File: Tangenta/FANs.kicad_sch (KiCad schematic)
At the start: 8 parts, among them M1 Fan_4pin, M2 Fan_4pin, Q3 BSS138

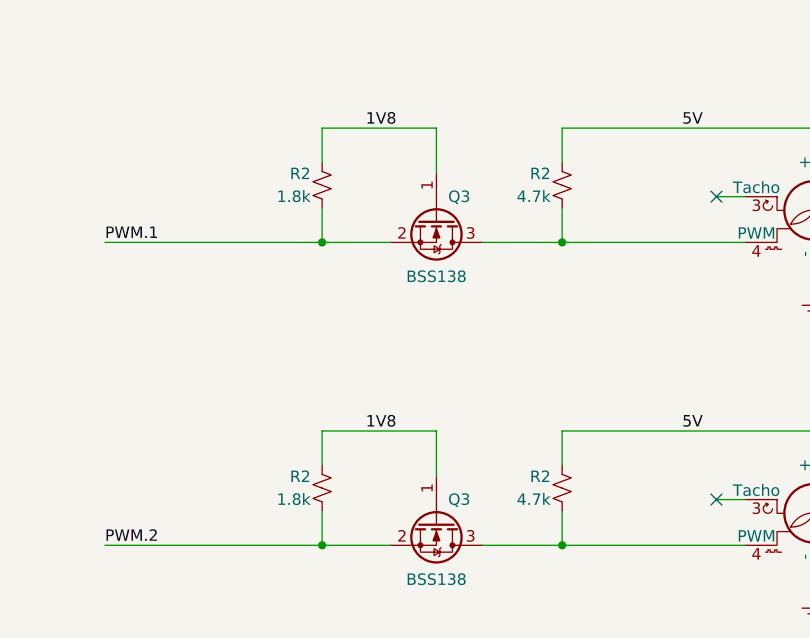
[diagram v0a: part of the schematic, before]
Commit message: initialize branch
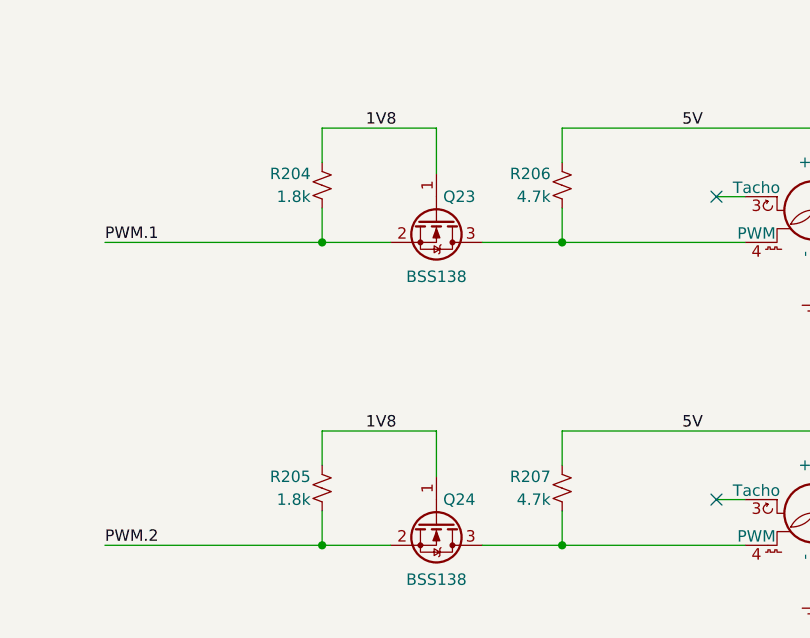
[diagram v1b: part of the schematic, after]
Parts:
- renumbered Q3 to Q23, Q3 to Q24, R2 to R204, R2 to R205, R2 to R206, R2 to R207
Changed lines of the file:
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@@
   (symbol (lib_id "CholaSymbolsPrjLib:R_Small_US") (at 127 111.76 180) (unit 1)
     (in_bom yes) (on_board yes) (dnp no)
-    (property "Reference" "R2" (at 125.73 110.49 0)
+    (property "Reference" "R205" (at 125.73 110.49 0)
       (effects (font (size 1.27 1.27)) (justify left))
     )
@@
     (instances
       (project "Tangenta"
-        (path "/358d1bcf-7599-4352-8c4d-baa18a5f09e6/8215796b-9611-4f43-bcc5-319f8414b8a6"
-          (reference "R2") (unit 1)
-        )
-        (path "/358d1bcf-7599-4352-8c4d-baa18a5f09e6/d6c05402-162e-441f-bed8-be7996260fb4"
-          (reference "R18") (unit 1)
-        )
-        (path "/358d1bcf-7599-4352-8c4d-baa18a5f09e6/b1871a4d-6a35-44e2-a9a2-9a4af684371d"
-          (reference "R26") (unit 1)
-        )
-        (path "/358d1bcf-7599-4352-8c4d-baa18a5f09e6/6a8c68b5-4a7d-449e-86f6-34ced6d1cb55"
-          (reference "R41") (unit 1)
-        )
-        (path "/358d1bcf-7599-4352-8c4d-baa18a5f09e6/db297b0b-35f2-4e86-892c-83973f1ac2db"
-          (reference "R41") (unit 1)
-        )
-        (path "/358d1bcf-7599-4352-8c4d-baa18a5f09e6/98e3b24f-9927-4339-b8fd-9deea91a522a"
-          (reference "R158") (unit 1)
-        )
         (path "/358d1bcf-7599-4352-8c4d-baa18a5f09e6/19b4ac3b-c2a1-43b1-8d7b-1ca5ac2c79ee"
           (reference "R205") (unit 1)
@@
   (symbol (lib_id "CholaSymbolsPrjLib:R_Small_US") (at 127 78.105 180) (unit 1)
     (in_bom yes) (on_board yes) (dnp no)
-    (property "Reference" "R2" (at 125.73 76.835 0)
+    (property "Reference" "R204" (at 125.73 76.835 0)
       (effects (font (size 1.27 1.27)) (justify left))
     )
@@
     (instances
       (project "Tangenta"
-        (path "/358d1bcf-7599-4352-8c4d-baa18a5f09e6/8215796b-9611-4f43-bcc5-319f8414b8a6"
-          (reference "R2") (unit 1)
-        )
-        (path "/358d1bcf-7599-4352-8c4d-baa18a5f09e6/d6c05402-162e-441f-bed8-be7996260fb4"
-          (reference "R18") (unit 1)
-        )
-        (path "/358d1bcf-7599-4352-8c4d-baa18a5f09e6/b1871a4d-6a35-44e2-a9a2-9a4af684371d"
-          (reference "R26") (unit 1)
-        )
-        (path "/358d1bcf-7599-4352-8c4d-baa18a5f09e6/6a8c68b5-4a7d-449e-86f6-34ced6d1cb55"
-          (reference "R41") (unit 1)
-        )
-        (path "/358d1bcf-7599-4352-8c4d-baa18a5f09e6/db297b0b-35f2-4e86-892c-83973f1ac2db"
-          (reference "R41") (unit 1)
-        )
-        (path "/358d1bcf-7599-4352-8c4d-baa18a5f09e6/98e3b24f-9927-4339-b8fd-9deea91a522a"
-          (reference "R158") (unit 1)
-        )
         (path "/358d1bcf-7599-4352-8c4d-baa18a5f09e6/19b4ac3b-c2a1-43b1-8d7b-1ca5ac2c79ee"
           (reference "R204") (unit 1)
@@
   (symbol (lib_id "CholaSymbolsPrjLib:BSS138") (at 139.7 115.57 270) (unit 1)
     (in_bom yes) (on_board yes) (dnp no)
-    (property "Reference" "Q3" (at 142.24 113.03 90)
+    (property "Reference" "Q24" (at 142.24 113.03 90)
       (effects (font (size 1.27 1.27)))
     )
@@
     (instances
       (project "Tangenta"
-        (path "/358d1bcf-7599-4352-8c4d-baa18a5f09e6/6a8c68b5-4a7d-449e-86f6-34ced6d1cb55"
-          (reference "Q3") (unit 1)
-        )
-        (path "/358d1bcf-7599-4352-8c4d-baa18a5f09e6/db297b0b-35f2-4e86-892c-83973f1ac2db"
-          (reference "Q5") (unit 1)
-        )
-        (path "/358d1bcf-7599-4352-8c4d-baa18a5f09e6/98e3b24f-9927-4339-b8fd-9deea91a522a"
-          (reference "Q10") (unit 1)
-        )
         (path "/358d1bcf-7599-4352-8c4d-baa18a5f09e6/19b4ac3b-c2a1-43b1-8d7b-1ca5ac2c79ee"
           (reference "Q24") (unit 1)
@@
   (symbol (lib_id "CholaSymbolsPrjLib:R_Small_US") (at 153.67 111.76 180) (unit 1)
     (in_bom yes) (on_board yes) (dnp no)
-    (property "Reference" "R2" (at 152.4 110.49 0)
+    (property "Reference" "R207" (at 152.4 110.49 0)
       (effects (font (size 1.27 1.27)) (justify left))
     )
@@
     (instances
       (project "Tangenta"
-        (path "/358d1bcf-7599-4352-8c4d-baa18a5f09e6/8215796b-9611-4f43-bcc5-319f8414b8a6"
-          (reference "R2") (unit 1)
-        )
-        (path "/358d1bcf-7599-4352-8c4d-baa18a5f09e6/d6c05402-162e-441f-bed8-be7996260fb4"
-          (reference "R18") (unit 1)
-        )
-        (path "/358d1bcf-7599-4352-8c4d-baa18a5f09e6/b1871a4d-6a35-44e2-a9a2-9a4af684371d"
-          (reference "R28") (unit 1)
-        )
-        (path "/358d1bcf-7599-4352-8c4d-baa18a5f09e6/db297b0b-35f2-4e86-892c-83973f1ac2db"
-          (reference "R28") (unit 1)
-        )
-        (path "/358d1bcf-7599-4352-8c4d-baa18a5f09e6/98e3b24f-9927-4339-b8fd-9deea91a522a"
-          (reference "R159") (unit 1)
-        )
         (path "/358d1bcf-7599-4352-8c4d-baa18a5f09e6/19b4ac3b-c2a1-43b1-8d7b-1ca5ac2c79ee"
           (reference "R207") (unit 1)
@@
   (symbol (lib_id "CholaSymbolsPrjLib:R_Small_US") (at 153.67 78.105 180) (unit 1)
     (in_bom yes) (on_board yes) (dnp no)
-    (property "Reference" "R2" (at 152.4 76.835 0)
+    (property "Reference" "R206" (at 152.4 76.835 0)
       (effects (font (size 1.27 1.27)) (justify left))
     )
@@
     (instances
       (project "Tangenta"
-        (path "/358d1bcf-7599-4352-8c4d-baa18a5f09e6/8215796b-9611-4f43-bcc5-319f8414b8a6"
-          (reference "R2") (unit 1)
-        )
-        (path "/358d1bcf-7599-4352-8c4d-baa18a5f09e6/d6c05402-162e-441f-bed8-be7996260fb4"
-          (reference "R18") (unit 1)
-        )
-        (path "/358d1bcf-7599-4352-8c4d-baa18a5f09e6/b1871a4d-6a35-44e2-a9a2-9a4af684371d"
-          (reference "R28") (unit 1)
-        )
-        (path "/358d1bcf-7599-4352-8c4d-baa18a5f09e6/db297b0b-35f2-4e86-892c-83973f1ac2db"
-          (reference "R28") (unit 1)
-        )
-        (path "/358d1bcf-7599-4352-8c4d-baa18a5f09e6/98e3b24f-9927-4339-b8fd-9deea91a522a"
-          (reference "R159") (unit 1)
-        )
         (path "/358d1bcf-7599-4352-8c4d-baa18a5f09e6/19b4ac3b-c2a1-43b1-8d7b-1ca5ac2c79ee"
           (reference "R206") (unit 1)
@@
   (symbol (lib_id "power:GNDREF") (at 181.61 123.825 0) (unit 1)
     (in_bom yes) (on_board yes) (dnp no) (fields_autoplaced)
-    (property "Reference" "#PWR030" (at 181.61 130.175 0)
+    (property "Reference" "#PWR0112" (at 181.61 130.175 0)
       (effects (font (size 1.27 1.27)) hide)
     )
@@
     (instances
       (project "Tangenta"
-        (path "/358d1bcf-7599-4352-8c4d-baa18a5f09e6/b1871a4d-6a35-44e2-a9a2-9a4af684371d"
-          (reference "#PWR030") (unit 1)
-        )
-        (path "/358d1bcf-7599-4352-8c4d-baa18a5f09e6/f1c5822c-e7b8-40ae-bab0-71fd1c2cfc7c"
-          (reference "#PWR035") (unit 1)
-        )
-        (path "/358d1bcf-7599-4352-8c4d-baa18a5f09e6/98e3b24f-9927-4339-b8fd-9deea91a522a"
-          (reference "#PWR076") (unit 1)
-        )
         (path "/358d1bcf-7599-4352-8c4d-baa18a5f09e6/19b4ac3b-c2a1-43b1-8d7b-1ca5ac2c79ee"
           (reference "#PWR0112") (unit 1)
@@
   (symbol (lib_id "power:GNDREF") (at 181.61 90.17 0) (unit 1)
     (in_bom yes) (on_board yes) (dnp no) (fields_autoplaced)
-    (property "Reference" "#PWR030" (at 181.61 96.52 0)
+    (property "Reference" "#PWR0111" (at 181.61 96.52 0)
       (effects (font (size 1.27 1.27)) hide)
     )
@@
     (instances
       (project "Tangenta"
-        (path "/358d1bcf-7599-4352-8c4d-baa18a5f09e6/b1871a4d-6a35-44e2-a9a2-9a4af684371d"
-          (reference "#PWR030") (unit 1)
-        )
-        (path "/358d1bcf-7599-4352-8c4d-baa18a5f09e6/f1c5822c-e7b8-40ae-bab0-71fd1c2cfc7c"
-          (reference "#PWR035") (unit 1)
-        )
-        (path "/358d1bcf-7599-4352-8c4d-baa18a5f09e6/98e3b24f-9927-4339-b8fd-9deea91a522a"
-          (reference "#PWR076") (unit 1)
-        )
         (path "/358d1bcf-7599-4352-8c4d-baa18a5f09e6/19b4ac3b-c2a1-43b1-8d7b-1ca5ac2c79ee"
           (reference "#PWR0111") (unit 1)
@@
   (symbol (lib_id "CholaSymbolsPrjLib:BSS138") (at 139.7 81.915 270) (unit 1)
     (in_bom yes) (on_board yes) (dnp no)
-    (property "Reference" "Q3" (at 142.24 79.375 90)
+    (property "Reference" "Q23" (at 142.24 79.375 90)
       (effects (font (size 1.27 1.27)))
     )
@@
     (instances
       (project "Tangenta"
-        (path "/358d1bcf-7599-4352-8c4d-baa18a5f09e6/6a8c68b5-4a7d-449e-86f6-34ced6d1cb55"
-          (reference "Q3") (unit 1)
-        )
-        (path "/358d1bcf-7599-4352-8c4d-baa18a5f09e6/db297b0b-35f2-4e86-892c-83973f1ac2db"
-          (reference "Q5") (unit 1)
-        )
-        (path "/358d1bcf-7599-4352-8c4d-baa18a5f09e6/98e3b24f-9927-4339-b8fd-9deea91a522a"
-          (reference "Q10") (unit 1)
-        )
         (path "/358d1bcf-7599-4352-8c4d-baa18a5f09e6/19b4ac3b-c2a1-43b1-8d7b-1ca5ac2c79ee"
           (reference "Q23") (unit 1)
@@
   (symbol (lib_id "power:GNDREF") (at 43.18 25.4 90) (unit 1)
     (in_bom yes) (on_board yes) (dnp no) (fields_autoplaced)
-    (property "Reference" "#PWR030" (at 49.53 25.4 0)
+    (property "Reference" "#PWR0110" (at 49.53 25.4 0)
       (effects (font (size 1.27 1.27)) hide)
     )
@@
     (instances
       (project "Tangenta"
-        (path "/358d1bcf-7599-4352-8c4d-baa18a5f09e6/b1871a4d-6a35-44e2-a9a2-9a4af684371d"
-          (reference "#PWR030") (unit 1)
-        )
-        (path "/358d1bcf-7599-4352-8c4d-baa18a5f09e6/f1c5822c-e7b8-40ae-bab0-71fd1c2cfc7c"
-          (reference "#PWR035") (unit 1)
-        )
-        (path "/358d1bcf-7599-4352-8c4d-baa18a5f09e6/98e3b24f-9927-4339-b8fd-9deea91a522a"
-          (reference "#PWR076") (unit 1)
-        )
         (path "/358d1bcf-7599-4352-8c4d-baa18a5f09e6/19b4ac3b-c2a1-43b1-8d7b-1ca5ac2c79ee"
           (reference "#PWR0110") (unit 1)
